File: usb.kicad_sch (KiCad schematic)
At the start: 14 parts, among them J4 Conn_01x05, U1 CH334R, Y1 12Mhz

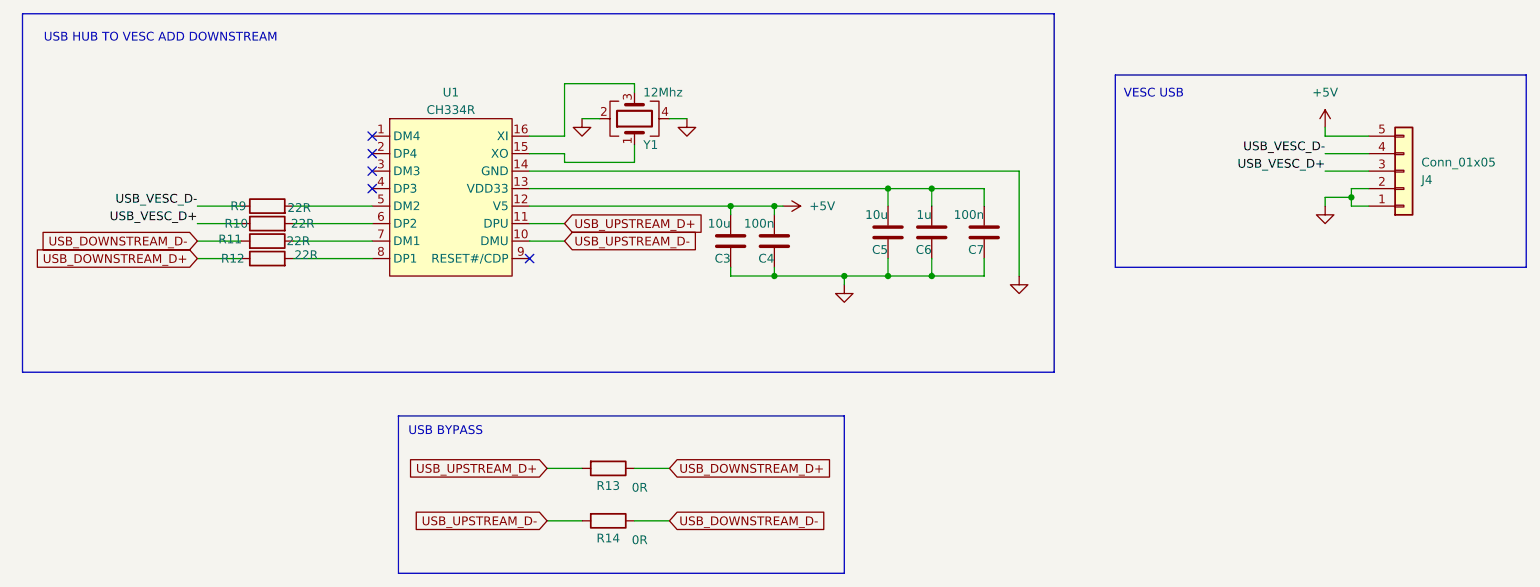
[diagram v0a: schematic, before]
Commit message: rev v3 tiny
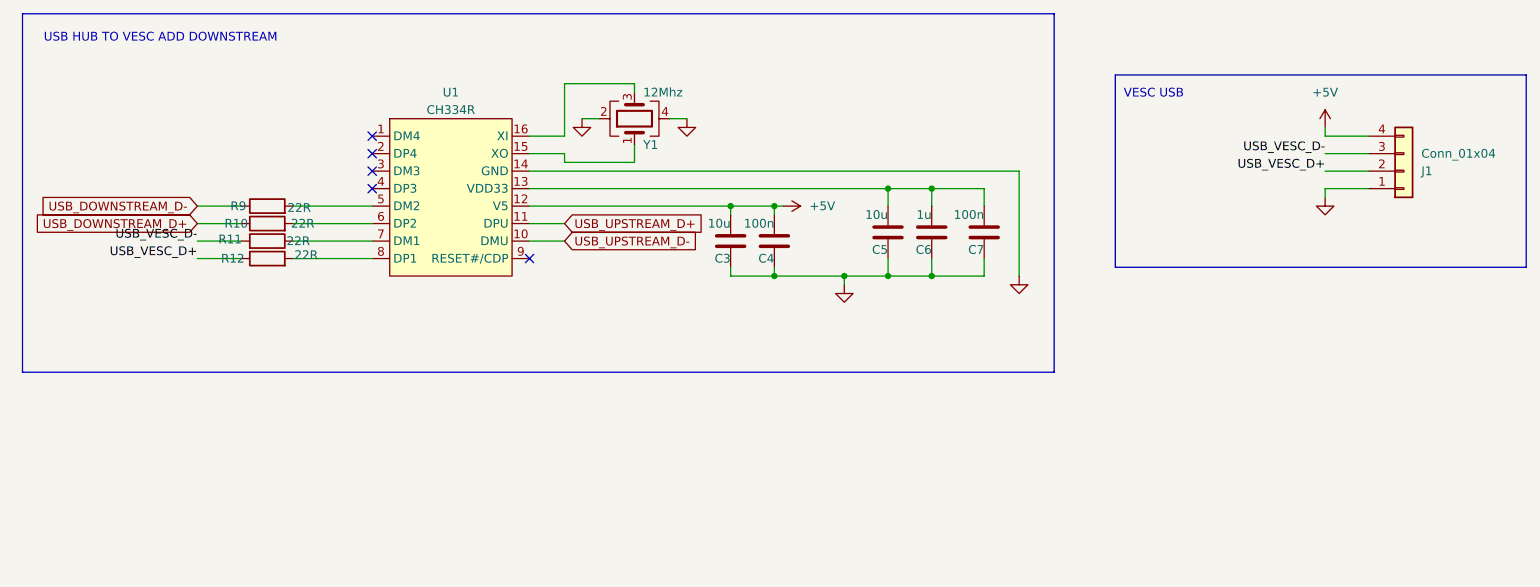
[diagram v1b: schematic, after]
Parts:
- removed J4: Conn_01x05, Connector_JST:JST_XH_B5B-XH-A_1x05_P2.50mm_Vertical, symbol Connector_Generic:Conn_01x05
- removed R13, R14: 0R, Resistor_SMD:R_0603_1608Metric, symbol Device:R
- added J1: Conn_01x04, Connector_JST:JST_XH_B4B-XH-A_1x04_P2.50mm_Vertical, symbol Connector_Generic:Conn_01x04
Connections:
- net +5V: now also J1.4 (Pin_4)
- net GND: now also J1.1 (Pin_1)
- net USB_DOWNSTREAM_D+: now also R10.1; no longer R12.1
- net USB_DOWNSTREAM_D-: now also R9.1; no longer R11.2
- net USB_VESC_D+: now also R12.1, J1.2 (Pin_2); no longer R10.1
- net USB_VESC_D-: now also R11.2, J1.3 (Pin_3); no longer R9.1
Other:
- note removed: "USB BYPASS"

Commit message: fix chinczyk funckup
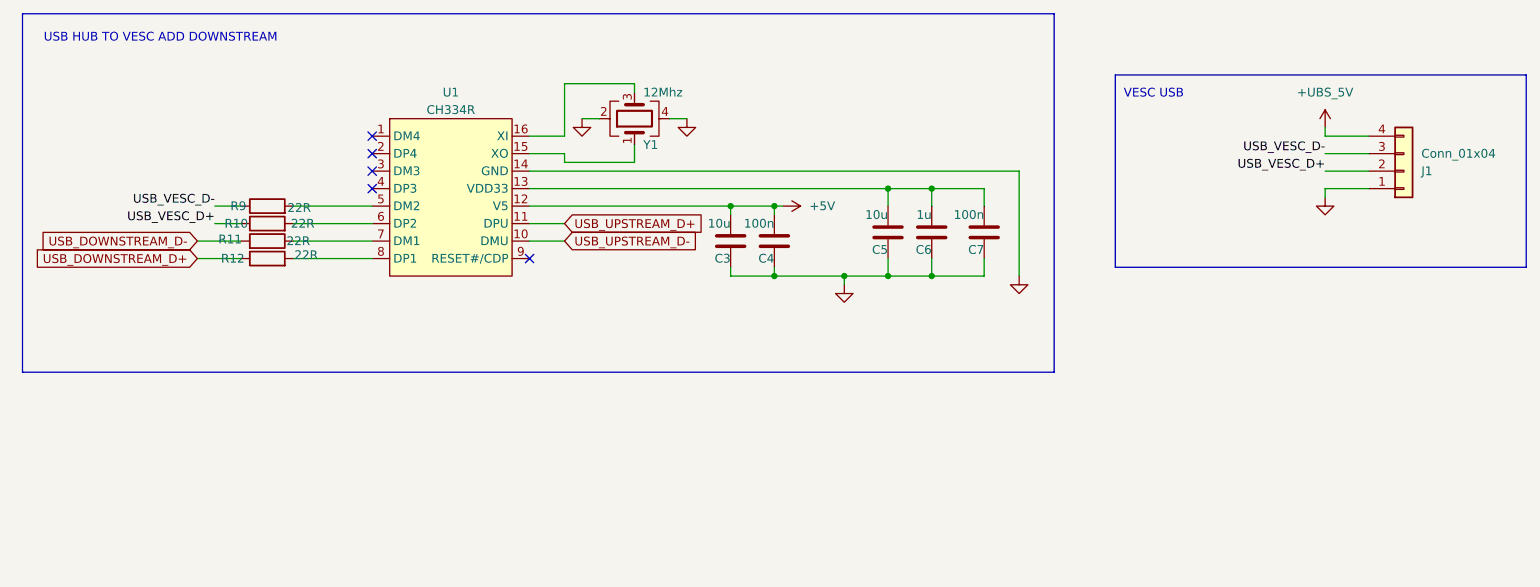
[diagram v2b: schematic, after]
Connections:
- net +5V: no longer J1.4 (Pin_4)
- net USB_DOWNSTREAM_D+: now also R12.1; no longer R10.1
- net USB_DOWNSTREAM_D-: now also R11.2; no longer R9.1
- net USB_VESC_D+: now also R10.1; no longer R12.1
- net USB_VESC_D-: now also R9.1; no longer R11.2
- new net +UBS_5V: J1.4 (Pin_4)
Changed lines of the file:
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@@
 	(wire
 		(pts
-			(xy 50.8 76.2) (xy 57.15 76.2)
+			(xy 53.34 76.2) (xy 57.15 76.2)
 		)
 		(stroke
@@
 	(wire
 		(pts
-			(xy 50.8 73.66) (xy 57.15 73.66)
+			(xy 53.34 73.66) (xy 57.15 73.66)
 		)
 		(stroke
@@
 	)
 	(label "USB_VESC_D+"
-		(at 50.8 81.28 180)
+		(at 53.34 76.2 180)
 		(effects
 			(font
@@
 	)
 	(label "USB_VESC_D-"
-		(at 50.8 78.74 180)
+		(at 53.34 73.66 180)
 		(effects
 			(font
@@
 			)
 			(justify right bottom)
-		)
-	)
-	(global_label "USB_DOWNSTREAM_D+"
-		(shape input)
-		(at 50.8 76.2 180)
-		(fields_autoplaced yes)
-		(effects
-			(font
-				(size 1.27 1.27)
-			)
-			(justify right)
-		)
-		(property "Intersheetrefs" "${INTERSHEET_REFS}"
-			(at 26.7087 76.2 0)
-			(effects
-				(font
-					(size 1.27 1.27)
-				)
-				(justify right)
-				(hide yes)
-			)
 		)
 	)
@@
 	(global_label "USB_DOWNSTREAM_D-"
 		(shape input)
-		(at 50.8 73.66 180)
+		(at 50.8 78.74 180)
 		(fields_autoplaced yes)
 		(effects
@@
 		)
 		(property "Intersheetrefs" "${INTERSHEET_REFS}"
-			(at 26.7087 73.66 0)
+			(at 26.7087 78.74 0)
+			(effects
+				(font
+					(size 1.27 1.27)
+				)
+				(justify right)
+				(hide yes)
+			)
+		)
+	)
+	(global_label "USB_DOWNSTREAM_D+"
+		(shape input)
+		(at 50.8 81.28 180)
+		(fields_autoplaced yes)
+		(effects
+			(font
+				(size 1.27 1.27)
+			)
+			(justify right)
+		)
+		(property "Intersheetrefs" "${INTERSHEET_REFS}"
+			(at 26.7087 81.28 0)
 			(effects
 				(font
@@
 			)
 		)
-		(property "Value" "+5V"
+		(property "Value" "+UBS_5V"
 			(at 214.63 57.15 0)
 			(effects
